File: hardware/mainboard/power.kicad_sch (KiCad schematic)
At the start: 18 parts

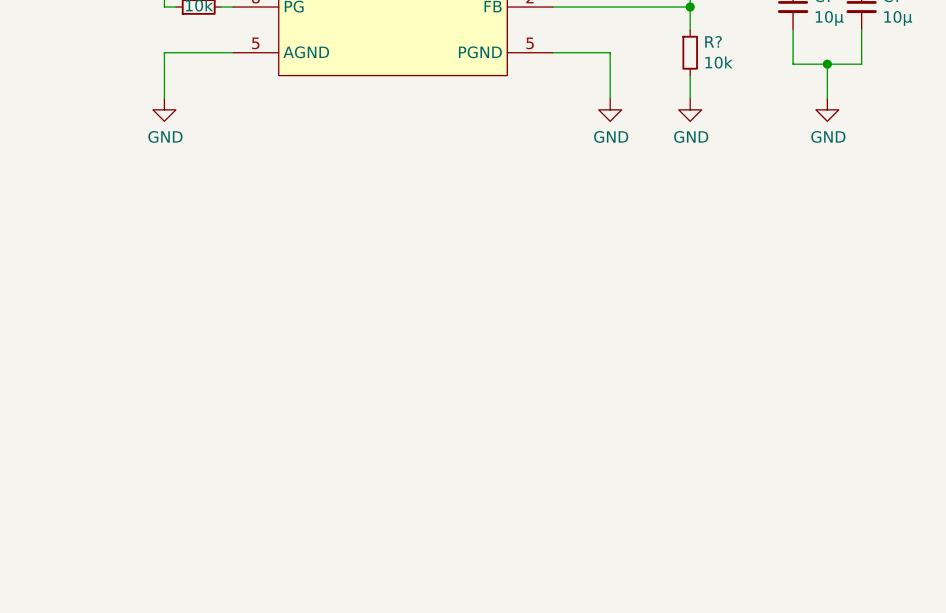
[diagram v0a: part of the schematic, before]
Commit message: More stuff
Signed-off-by: David Shah <dave@ds0.me>
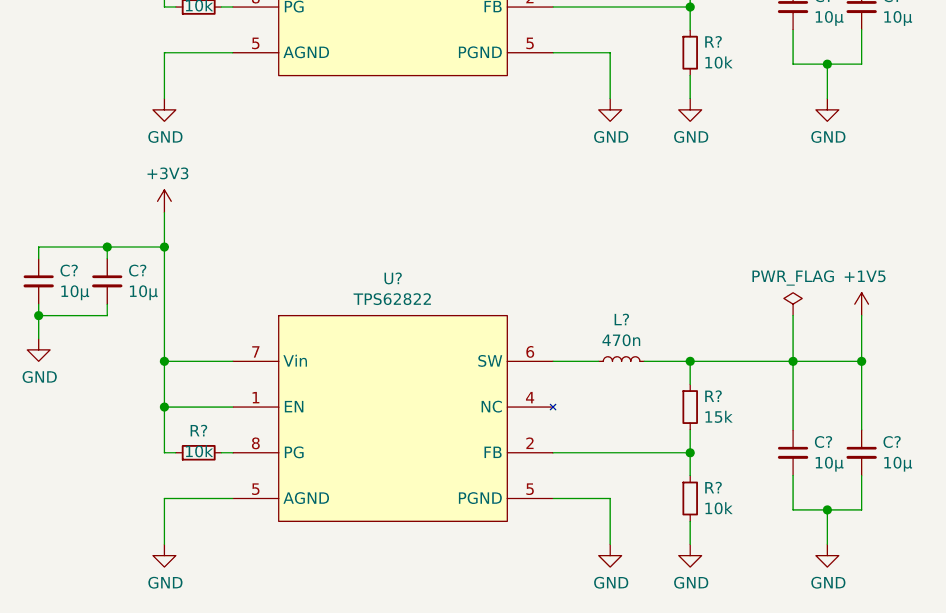
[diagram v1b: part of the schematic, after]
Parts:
- added C? (x4): 10µ, symbol Device:C_Small
- added L?: 470n, symbol Device:L_Small
- added R? (x2): 10k, symbol Device:R_Small
- added R?: 15k, symbol Device:R_Small
- added U?: TPS62822, symbol meowality:TPS62823
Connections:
- net +3V3: now also C?.1, C?.1, R?.1, U?.1 (EN), U?.7 (Vin)
- net GND: now also C?.2, C?.2, C?.2, C?.2, R?.2, U?.5 (PGND)
- new net: L?.1, U?.6 (SW)
- new net: R?.1, R?.2, U?.2 (FB)
- new net: R?.2, U?.8 (PG)
- new net +1V5: C?.1, C?.1, L?.2, R?.1
